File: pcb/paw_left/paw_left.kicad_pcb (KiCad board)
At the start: 2 copper layers, 140 x 96 mm, 44 parts, among them U1 Nice_Nano_V2

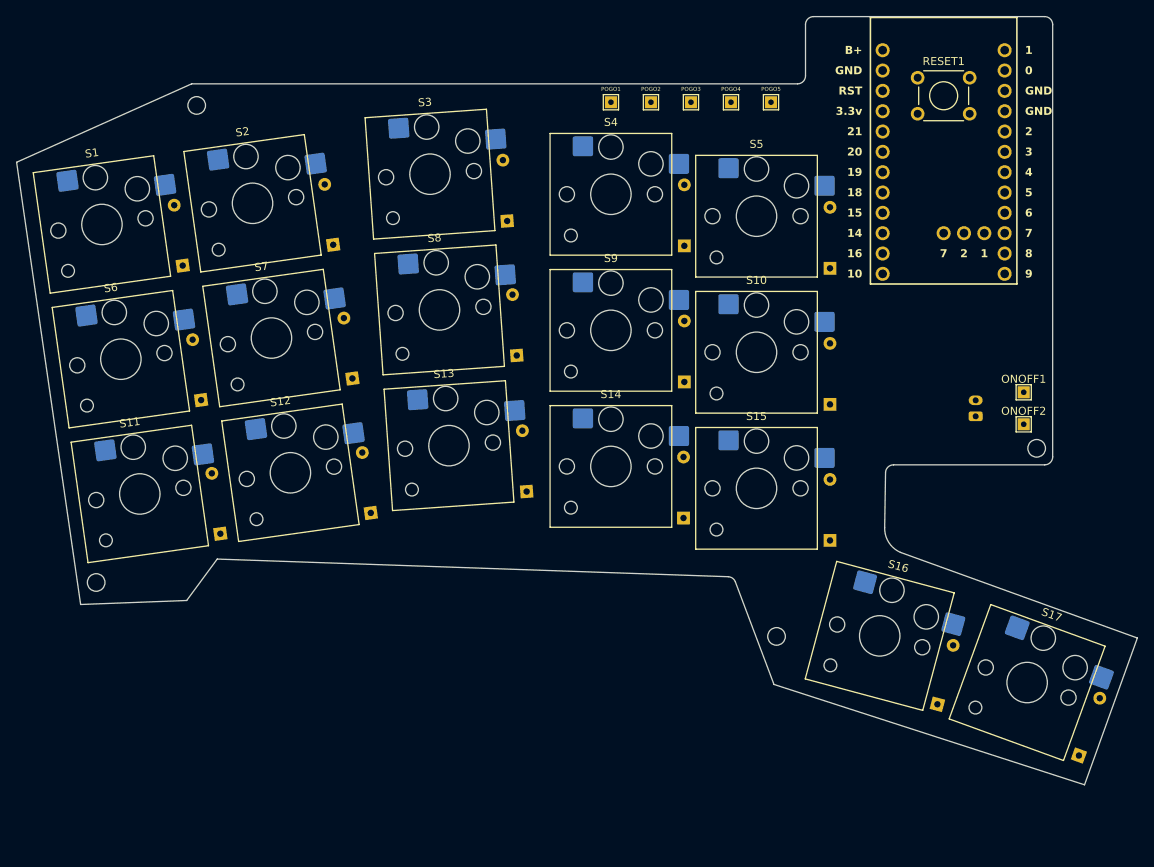
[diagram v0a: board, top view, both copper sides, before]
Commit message: Added right hand PCB
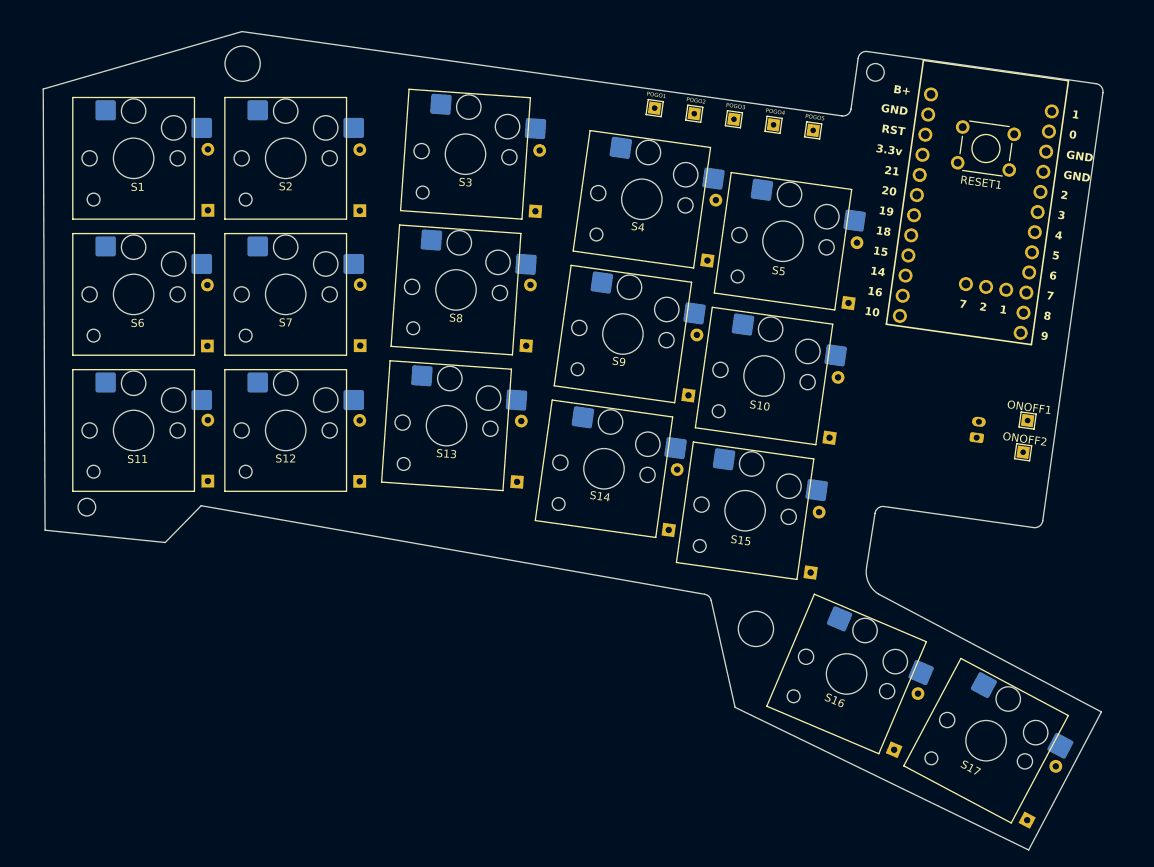
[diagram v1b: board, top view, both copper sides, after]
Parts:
- moved RESET1 16.2 mm to (189.7, 143.8), turned to 172 degrees
- moved D17 10.3 mm to (191.9, 225.0), turned to 62 degrees
- moved S1 9.16 mm to (80.3, 142.3), turned to 0 degrees
- moved S17 8.90 mm to (186.8, 215.1), turned to -28 degrees
- moved S6 8.25 mm to (80.3, 159.3), turned to 0 degrees
- moved S11 7.97 mm to (80.3, 176.3), turned to 0 degrees
- moved D16 7.84 mm to (175.3, 216.2), turned to 67 degrees
- moved U1 7.62 mm to (185.5, 149.0), turned to 172 degrees
- moved D1 7.59 mm to (89.6, 148.8), turned to 90 degrees
- moved S2 6.98 mm to (99.3, 142.3), turned to 0 degrees
- moved D6 6.80 mm to (89.5, 165.8), turned to 90 degrees
- moved D11 6.76 mm to (89.6, 182.7), turned to 90 degrees
- moved POGO5 6.34 mm to (165.2, 138.8), turned to -8 degrees
- moved S16 6.31 mm to (169.4, 206.8), turned to -23 degrees
- moved POGO4 6.02 mm to (160.2, 138.2), turned to -8 degrees
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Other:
- board size 140 x 96 mm -> 132.4 x 102.2 mm
